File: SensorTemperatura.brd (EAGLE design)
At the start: 68.6 x 54.9 mm, 18 parts, among them IC1 MAX481CPA, IC2 MEGA8-P, Q1 16mhz

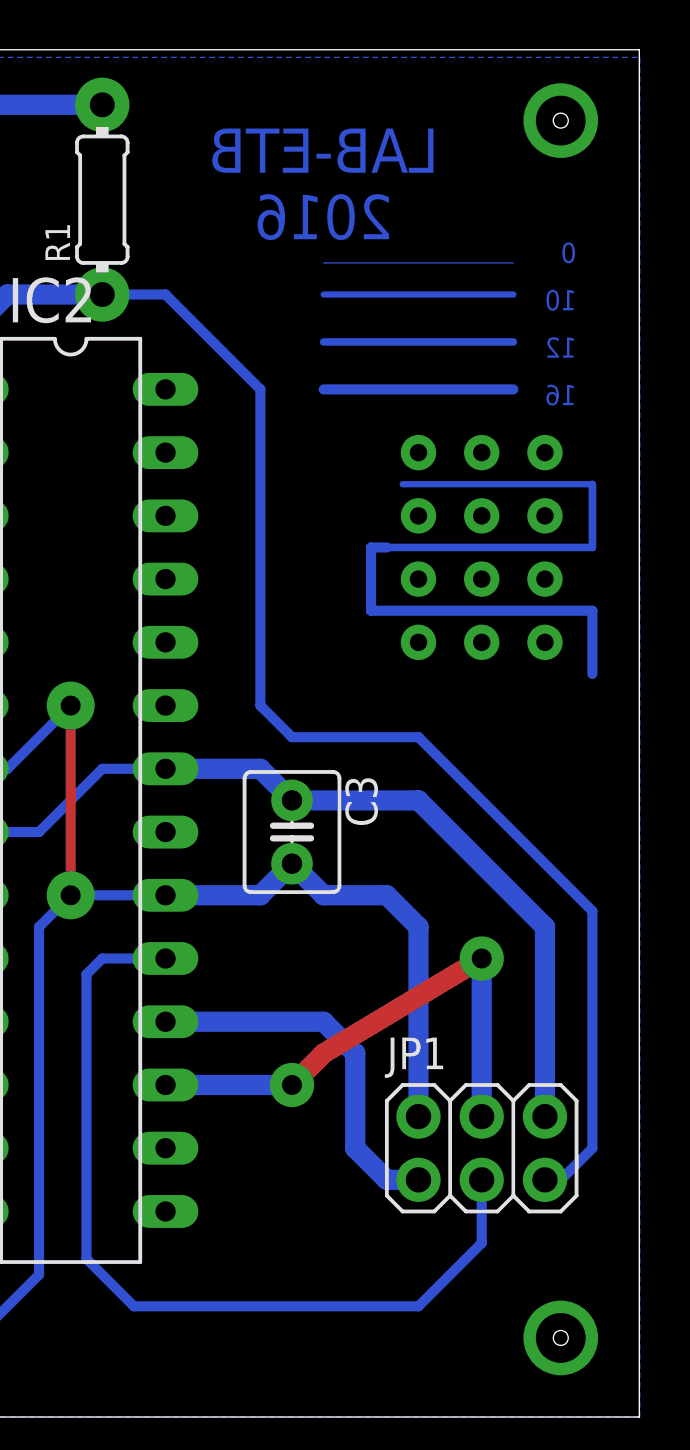
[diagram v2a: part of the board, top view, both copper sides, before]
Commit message: FIX
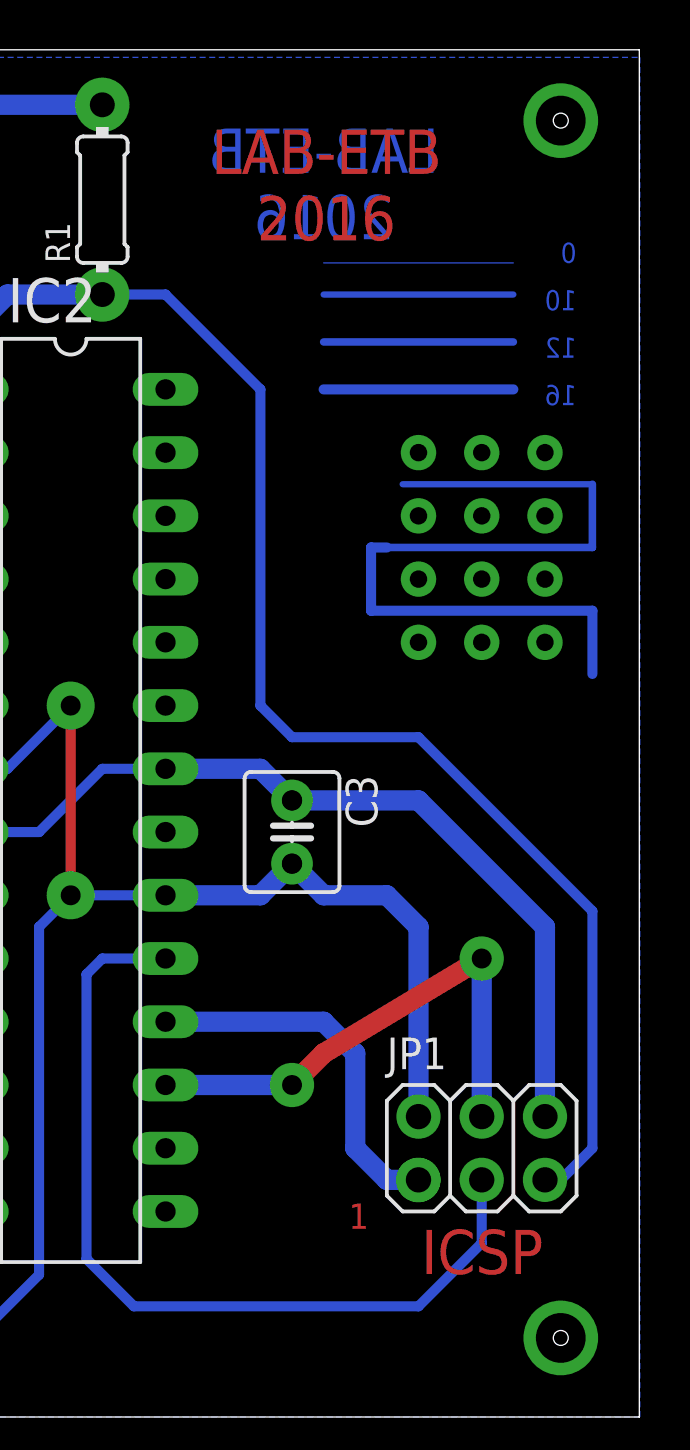
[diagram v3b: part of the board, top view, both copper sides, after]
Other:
- board text added: "1"
- board text added: "ICSP"
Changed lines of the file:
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@@
 <setting verticaltext="up"/>
 </settings>
-<grid distance="25" unitdist="mil" unit="mil" style="lines" multiple="1" display="no" altdistance="0.025" altunitdist="inch" altunit="inch"/>
+<grid distance="0.000123031496" unitdist="mil" unit="mil" style="lines" multiple="1" display="no" altdistance="0.025" altunitdist="inch" altunit="inch"/>
 <layers>
-<layer number="1" name="Top" color="4" fill="1" visible="no" active="yes"/>
+<layer number="1" name="Top" color="4" fill="1" visible="yes" active="yes"/>
 <layer number="2" name="Route2" color="1" fill="3" visible="no" active="no"/>
 <layer number="3" name="Route3" color="4" fill="3" visible="no" active="no"/>
@@
 <layer number="14" name="Route14" color="1" fill="6" visible="no" active="no"/>
 <layer number="15" name="Route15" color="4" fill="6" visible="no" active="no"/>
-<layer number="16" name="Bottom" color="1" fill="1" visible="yes" active="yes"/>
+<layer number="16" name="Bottom" color="1" fill="1" visible="no" active="yes"/>
 <layer number="17" name="Pads" color="2" fill="1" visible="yes" active="yes"/>
 <layer number="18" name="Vias" color="2" fill="1" visible="yes" active="yes"/>
-<layer number="19" name="Unrouted" color="6" fill="1" visible="yes" active="yes"/>
+<layer number="19" name="Unrouted" color="6" fill="1" visible="no" active="yes"/>
 <layer number="20" name="Dimension" color="15" fill="1" visible="yes" active="yes"/>
-<layer number="21" name="tPlace" color="7" fill="1" visible="no" active="yes"/>
-<layer number="22" name="bPlace" color="7" fill="1" visible="no" active="yes"/>
+<layer number="21" name="tPlace" color="7" fill="1" visible="yes" active="yes"/>
+<layer number="22" name="bPlace" color="7" fill="1" visible="yes" active="yes"/>
 <layer number="23" name="tOrigins" color="15" fill="1" visible="no" active="yes"/>
 <layer number="24" name="bOrigins" color="15" fill="1" visible="no" active="yes"/>
-<layer number="25" name="tNames" color="7" fill="1" visible="no" active="yes"/>
-<layer number="26" name="bNames" color="7" fill="1" visible="no" active="yes"/>
+<layer number="25" name="tNames" color="7" fill="1" visible="yes" active="yes"/>
+<layer number="26" name="bNames" color="7" fill="1" visible="yes" active="yes"/>
 <layer number="27" name="tValues" color="7" fill="1" visible="no" active="yes"/>
 <layer number="28" name="bValues" color="7" fill="1" visible="no" active="yes"/>
@@
 <layer number="43" name="vRestrict" color="2" fill="10" visible="no" active="yes"/>
 <layer number="44" name="Drills" color="7" fill="1" visible="no" active="yes"/>
-<layer number="45" name="Holes" color="7" fill="1" visible="yes" active="yes"/>
+<layer number="45" name="Holes" color="7" fill="1" visible="no" active="yes"/>
 <layer number="46" name="Milling" color="3" fill="1" visible="no" active="yes"/>
 <layer number="47" name="Measures" color="7" fill="1" visible="no" active="yes"/>
 <layer number="48" name="Document" color="7" fill="1" visible="no" active="yes"/>
 <layer number="49" name="Reference" color="7" fill="1" visible="no" active="yes"/>
-<layer number="51" name="tDocu" color="7" fill="1" visible="no" active="yes"/>
+<layer number="51" name="tDocu" color="7" fill="1" visible="yes" active="yes"/>
 <layer number="52" name="bDocu" color="7" fill="1" visible="no" active="yes"/>
 <layer number="90" name="Modules" color="5" fill="1" visible="no" active="no"/>
@@
 <text x="73.66" y="54.61" size="0.8128" layer="16" rot="MR0">12</text>
 <text x="73.66" y="52.705" size="0.8128" layer="16" rot="MR0">16</text>
+<text x="63.612546875" y="59.327225" size="1.778" layer="1" align="bottom-center">LAB-ETB
+2016</text>
+<text x="69.869359375" y="17.807053125" size="1.778" layer="1" align="bottom-center">ICSP</text>
+<text x="64.909215625" y="19.622259375" size="1.016" layer="1" align="bottom-center">1</text>
 </plain>
 <attributes>
@@
 <wire x1="63.5" y1="53.34" x2="71.12" y2="53.34" width="0.4064" layer="16"/>
 </signal>
+<signal name="S$41">
+<via x="67.299015625" y="21.57885" extent="1-16" drill="0.6" diameter="1.778" shape="square"/>
+</signal>
 </signals>
